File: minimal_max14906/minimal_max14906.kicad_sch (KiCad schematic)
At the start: 102 parts, among them J1 CLP-114-02-G-D-BE, J10 TBP02R2-381-02BE, J11 TBP02R2-381-02BE, J12 CLP-103-02-G-D-BE, J2 TBP02R2-381-02BE, J3 TBP02R2-381-02BE, J4 CLP-102-02-G-D-BE, J5 CLP-102-02-G-D-BE, J6 CLP-102-02-G-D-BE, J7 CLP-102-02-G-D-BE, J8 CLP-102-02-G-D-BE, J9 CLP-102-02-G-D-BE, Q1 -60.0 V, Q2 -60.0 V, Q3 -60.0 V, Q4 -60.0 V, Q5 100 V, U1 ADUM1252AUA+, U2 MAX22441CAEE+, U3 MAX22442CAEE+, U4 ADUM1252AUA+, U5 MAX14906ATM+

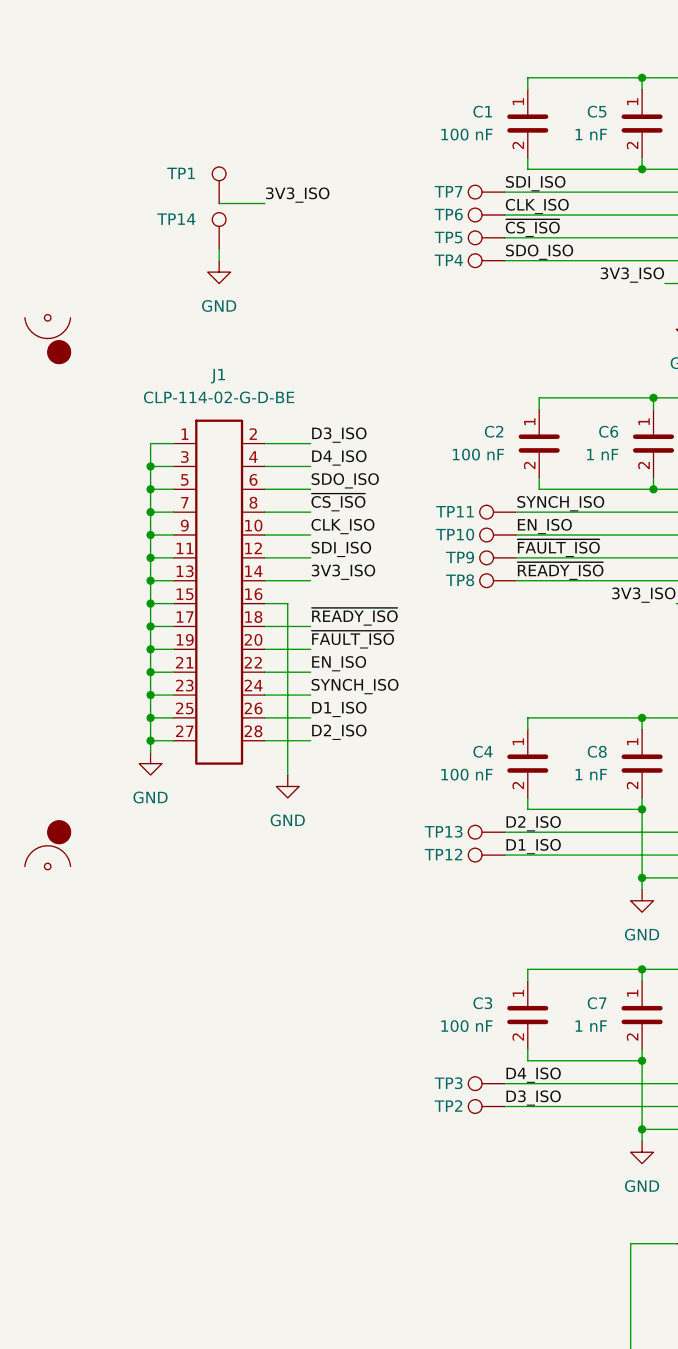
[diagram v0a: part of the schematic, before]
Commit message: development backup
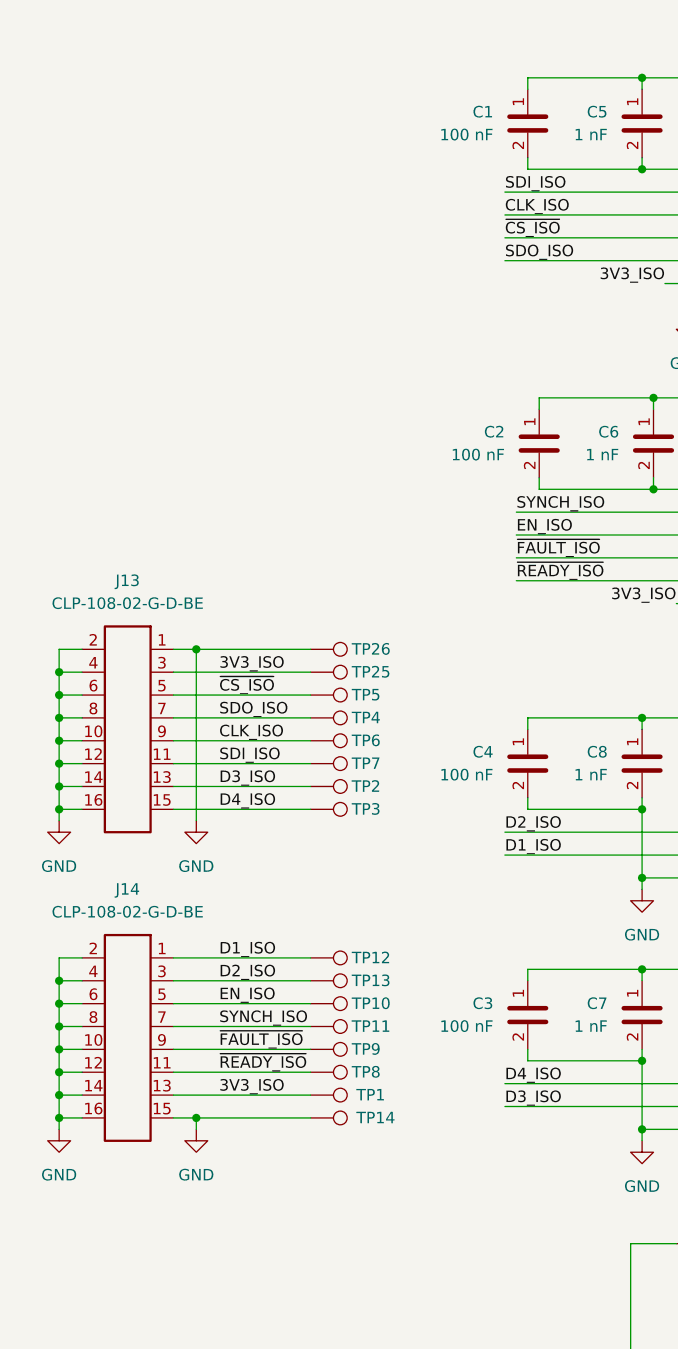
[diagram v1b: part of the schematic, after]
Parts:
- removed J1: CLP-114-02-G-D-BE, connector_footprints:CLP-114-02-G-D-BE, symbol UNITED_CONNECTORS_DATA_BASE:J_CLP-114-02-G-D-BE
- removed MB1: mouse-bite-midle-50mil-200mil, mouse_bite_footprints:mouse-bite-50mil-790mil, symbol UNITED_MOUSE_BITES_DATA_BASE:mouse-bite-50mil-790mil
- added J13, J14: CLP-108-02-G-D-BE, connector_footprints:CLP-108-02-G-D-BE, symbol UNITED_CONNECTORS_DATA_BASE:J_CLP-108-02-G-D-BE
- added TP25, TP26: TestPoint, test_point_footprints:TestPoint_THTPad_Castelated, symbol UNITED_TEST_POINTS:TestPoint_Castelated
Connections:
- net 3V3_ISO: now also J13.3, J14.13, TP25.1
- net CLK_ISO: now also J13.9
- net D1_ISO: now also J14.1
- net D2_ISO: now also J14.3
- net D3_ISO: now also J13.13
- net D4_ISO: now also J13.15
- net EN_ISO: now also J14.5
- net GND: now also J13.1, J13.10, J13.12, J13.14, J13.16, J13.2, J13.4, J13.6, J13.8, J14.10, J14.12, J14.14, J14.15, J14.16, J14.2, J14.4, J14.6, J14.8, TP26.1
- net SDI_ISO: now also J13.11
- net SDO_ISO: now also J13.7
- net SYNCH_ISO: now also J14.7
- net ~{CS_ISO}: now also J13.5
- net ~{FAULT_ISO}: now also J14.9
- net ~{READY_ISO}: now also J14.11
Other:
- moved on the sheet: TP1, TP10, TP11, TP12, TP13, TP14, TP2, TP3, TP4, TP5, TP6, TP7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
